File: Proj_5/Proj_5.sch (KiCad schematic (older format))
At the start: 0 parts

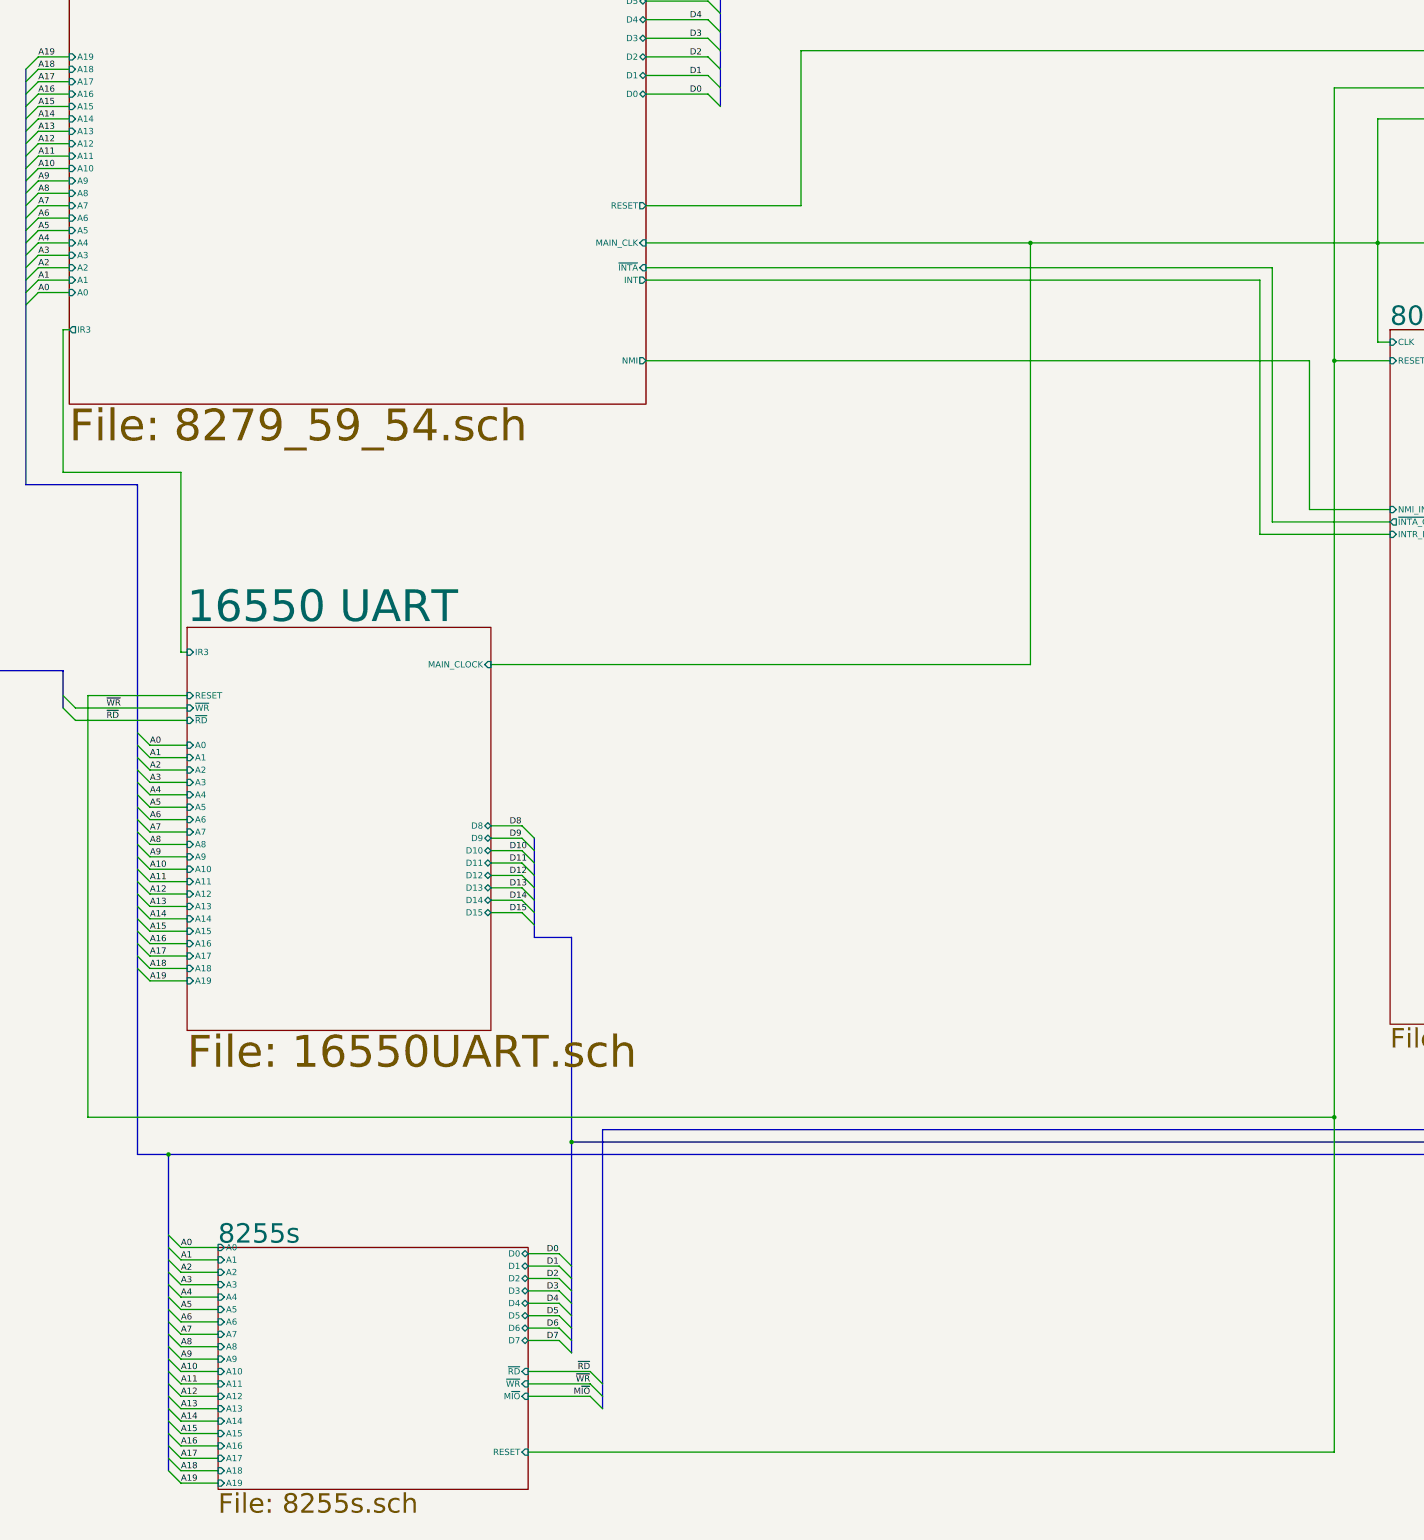
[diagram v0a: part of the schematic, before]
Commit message: Wires are Hell
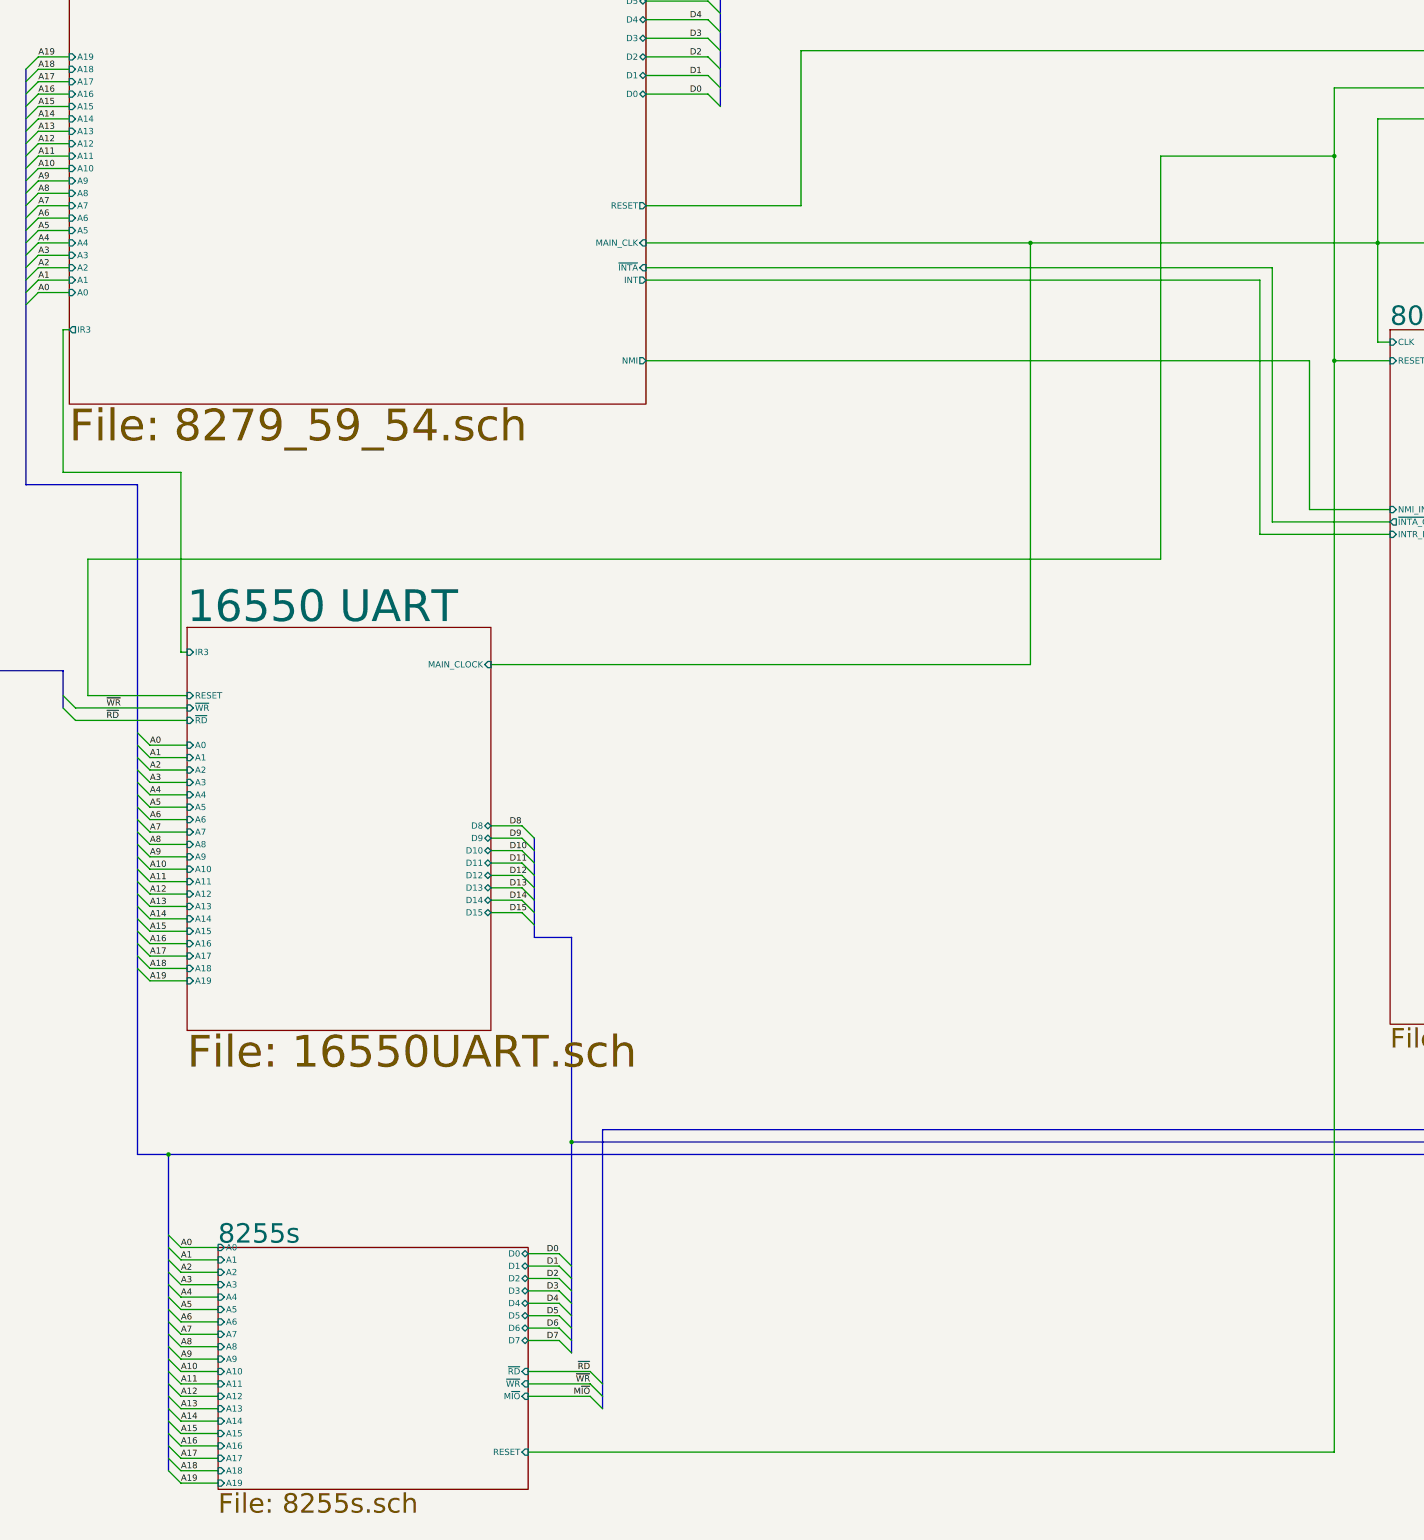
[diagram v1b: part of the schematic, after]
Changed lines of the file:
@@
 	14800 2950 13650 2950
 Wire Wire Line
-	13650 2950 13650 5150
+	13650 2950 13650 3500
 Wire Wire Line
 	13650 5150 14100 5150
-Wire Wire Line
-	13650 5150 13650 11250
 Connection ~ 13650 5150
 Wire Wire Line
@@
 Connection ~ 4250 11550
 Wire Wire Line
-	13650 11250 3600 11250
-Wire Wire Line
-	3600 11250 3600 7850
-Wire Wire Line
 	3600 7850 4400 7850
-Connection ~ 13650 11250
-Wire Wire Line
-	13650 11250 13650 13950
 $Sheet
 S 25850 13500 2300 3800
@@
 Text Label 28250 9050 0    50   ~ 0
 D8
+Wire Wire Line
+	13650 5150 13650 13950
+Wire Wire Line
+	3600 7850 3600 6750
+Wire Wire Line
+	3600 6750 12250 6750
+Wire Wire Line
+	12250 6750 12250 3500
+Wire Wire Line
+	12250 3500 13650 3500
 Wire Bus Line
 	3400 7650 3400 7950
@@
 Wire Bus Line
 	23550 13350 23550 16250
+Connection ~ 13650 3500
+Wire Wire Line
+	13650 3500 13650 5150
 $EndSCHEMATC
